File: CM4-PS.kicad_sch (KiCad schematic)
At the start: 32 parts, among them J19 Barrel_Jack, Q1 DMP3013SFV-7, U16 AP64501SP-13

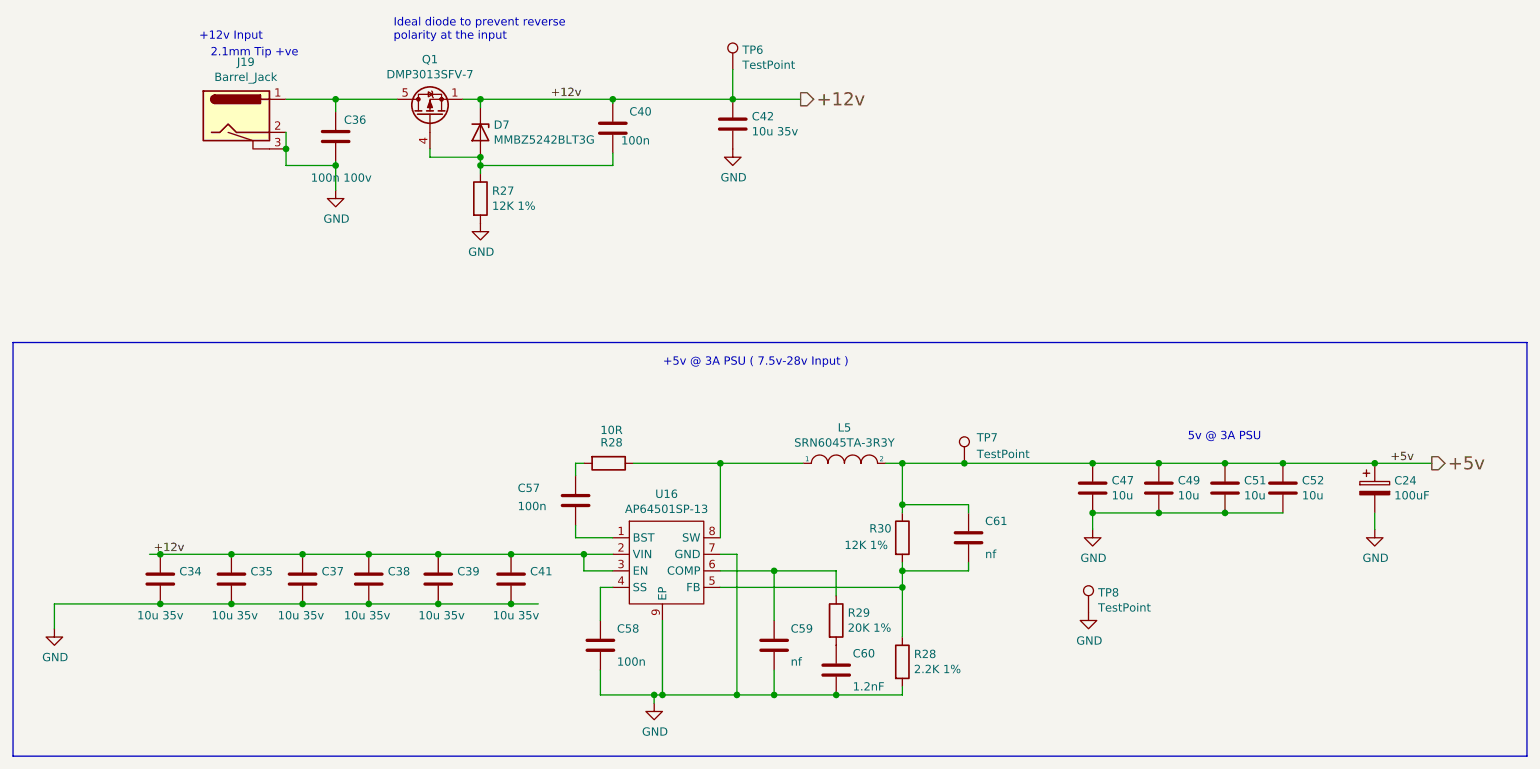
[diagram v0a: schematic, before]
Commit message: Need to fix ERC
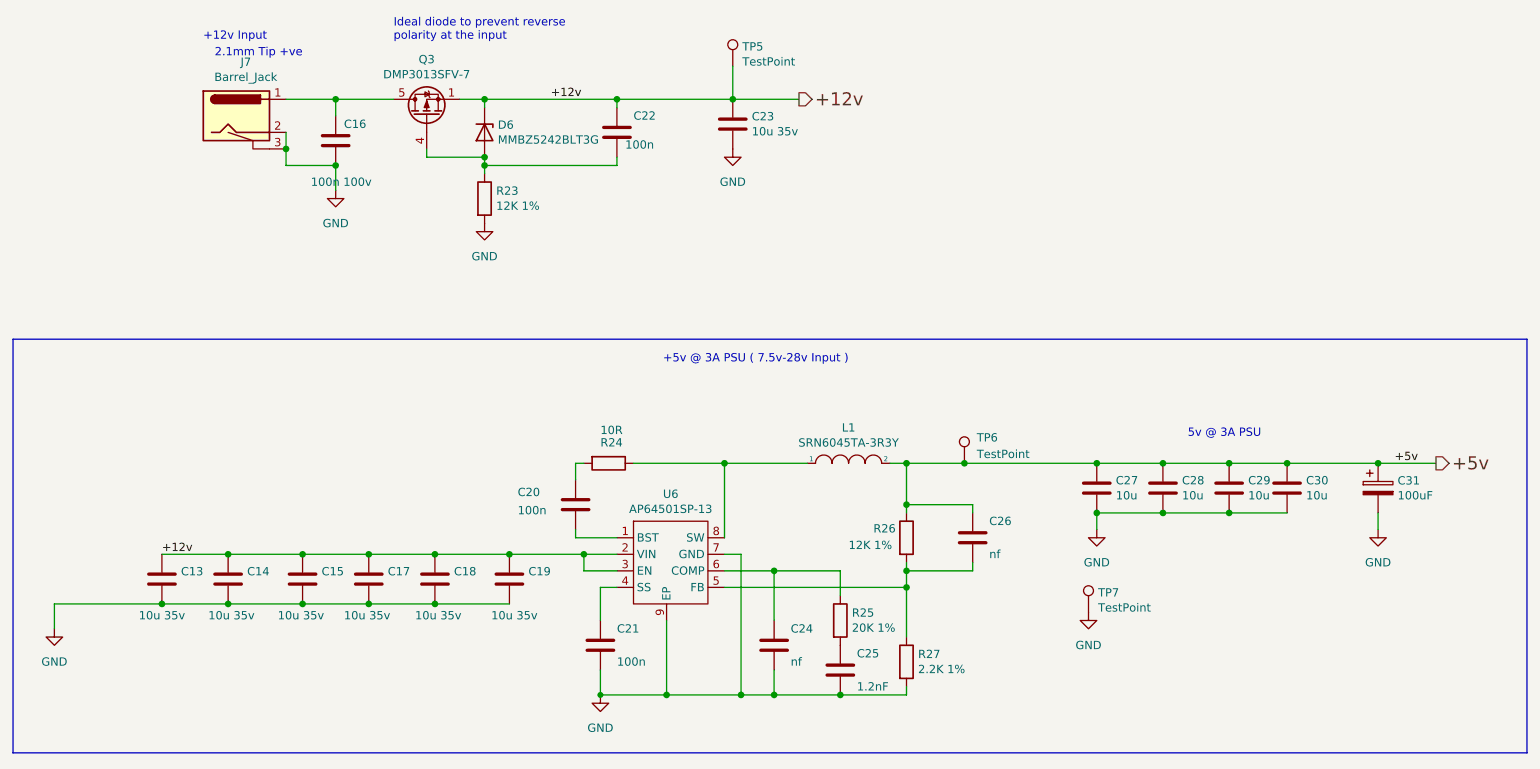
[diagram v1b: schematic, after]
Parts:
- removed R28: 2.2K 1%, Resistor_SMD:R_0402_1005Metric, symbol Device:R
- added R27: 2.2K 1%, Resistor_SMD:R_0402_1005Metric, symbol Device:R
- D6: renamed from D7; footprint Diode_SMD:D_SOT-23_ANK -> Package_TO_SOT_SMD:SOT-23
- renumbered C34 to C13, C35 to C14, C37 to C15, C36 to C16, C38 to C17, C39 to C18, C41 to C19, C57 to C20, C58 to C21, C40 to C22, C42 to C23, C59 to C24, C60 to C25, C61 to C26, C47 to C27, C49 to C28, C51 to C29, C52 to C30, C24 to C31, J19 to J7, L5 to L1, Q1 to Q3, R27 to R23, R28 to R24, R29 to R25, R30 to R26, TP6 to TP5, TP7 to TP6, TP8 to TP7, U16 to U6
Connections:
- net +12v: now also D6.3 (K); no longer D6.1 (K)
- net GND: now also R27.2
- net at C22.2, Q3.4 (G), R23.1: now also D6.1 (A); no longer D6.2 (A)
- net at C26.2, R26.2, U6.5 (FB): now also R27.1
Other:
- moved on the sheet: C14, C16, C18, C20, C22, C25, C26, C27, C28, C29, C30, C31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
